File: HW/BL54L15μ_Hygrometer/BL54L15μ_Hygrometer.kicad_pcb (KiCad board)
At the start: 2 copper layers, 25.4 x 25.4 mm, 21 parts, among them IC1 nrf54L 453-00223R, J1 Conn_Qwiic, J2 Conn_ARM_JTAG_SWD_10, U1 nPM2100-QEXX, U2 SHT4x, U3 STCC4-D-R3, U5 BME688, X1 32.768 kHz

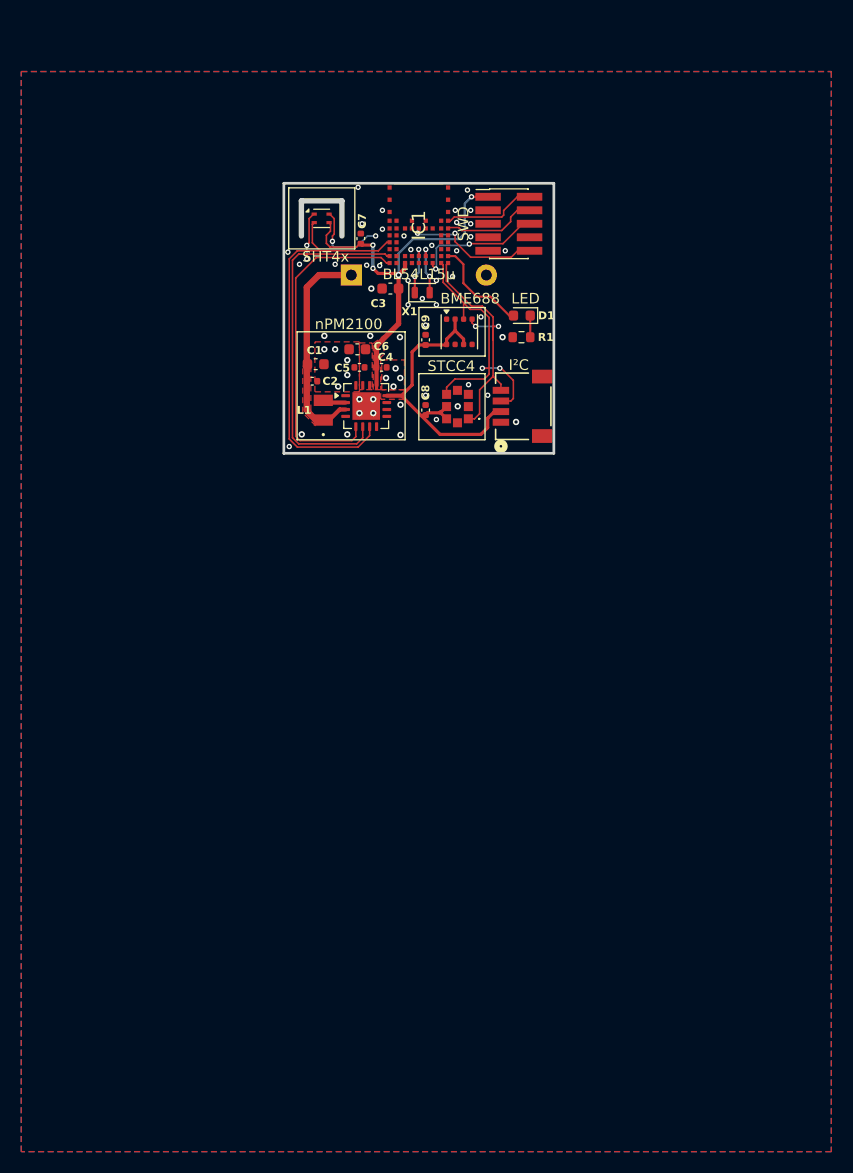
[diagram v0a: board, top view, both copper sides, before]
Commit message: BL54L15μ Hygrometer 2026v3
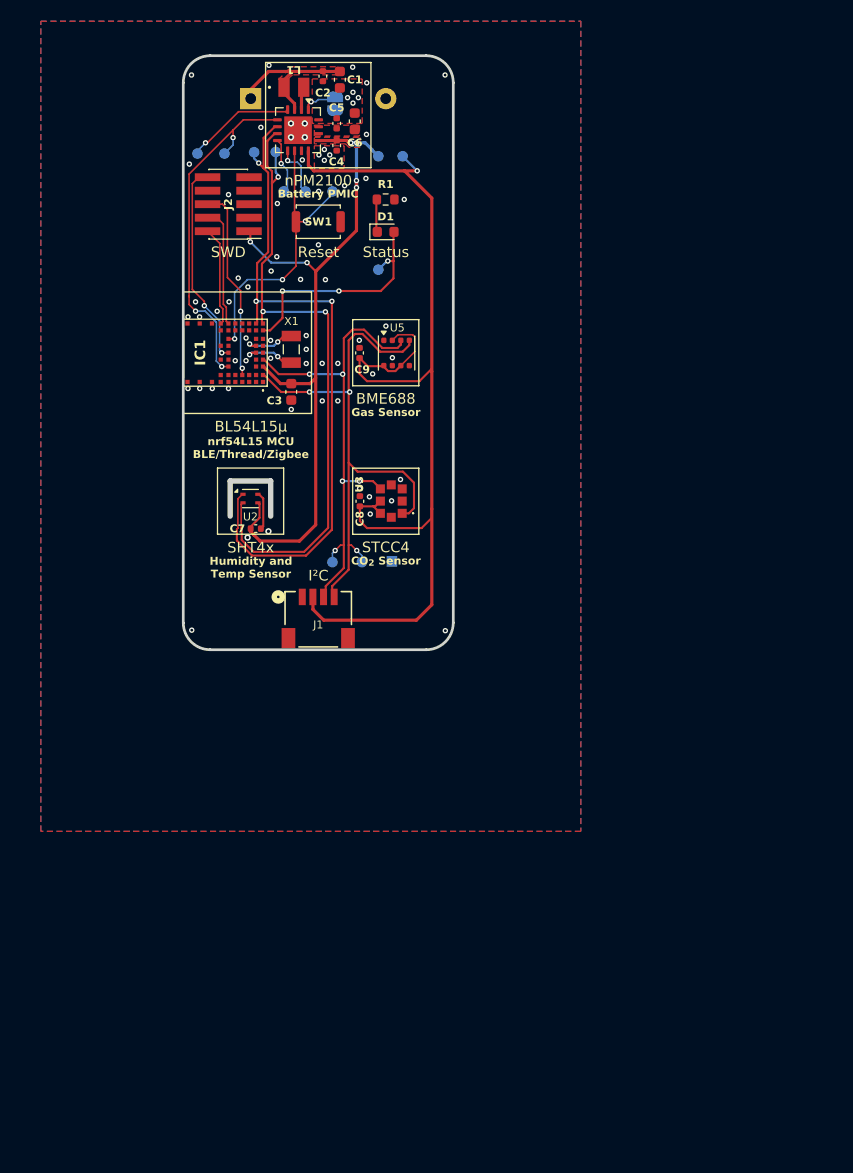
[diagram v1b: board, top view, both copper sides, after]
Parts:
- added JP1: VSET-GND, Jumper:SolderJumper-2_P1.3mm_Open_RoundedPad1.0x1.5mm, B.Cu at (103.9, 58.6)
- added SW1: Reset, Button_Switch_SMD:SW_Push_SPST_NO_Alps_SKRK, F.Cu at (102.3, 69.7)
- added TP1: VDD, TestPoint:TestPoint_Pad_D1.0mm, B.Cu at (108.0, 63.5)
- added TP10: PG/RESET, TestPoint:TestPoint_Pad_D1.0mm, B.Cu at (103.6, 66.8)
- added TP11: SYSGDEN, TestPoint:TestPoint_Pad_D1.0mm, B.Cu at (99.1, 66.8)
- added TP12: LED0, TestPoint:TestPoint_Pad_D1.0mm, B.Cu at (108.0, 74.2)
- added TP13: VDDSW, TestPoint:TestPoint_Pad_D1.0mm, B.Cu at (110.2, 63.5)
- added TP2: GND, TestPoint:TestPoint_Pad_1.0x1.0mm, B.Cu at (109.2, 101.6)
- added TP3: GPIO0/P0.01, TestPoint:TestPoint_Pad_D1.0mm, B.Cu at (93.5, 63.2)
- added TP4: GPIO1, TestPoint:TestPoint_Pad_D1.0mm, B.Cu at (101.1, 66.8)
- added TP5: SDA0/P1.14, TestPoint:TestPoint_Pad_D1.0mm, B.Cu at (96.3, 63.1)
- added TP6: SCL0/P1.04, TestPoint:TestPoint_Pad_D1.0mm, B.Cu at (98.3, 63.1)
- added TP7: SDA1/P1.06, TestPoint:TestPoint_Pad_D1.0mm, B.Cu at (103.6, 101.7)
- added TP8: SCL1/P1.08, TestPoint:TestPoint_Pad_D1.0mm, B.Cu at (106.4, 101.7)
- added TP9: SHPHLD, TestPoint:TestPoint_Pad_D1.0mm, B.Cu at (90.9, 63.2)
- BT1: footprint Battery:BatteryHolder_Keystone_2468_2xAAA -> BatteryHolder_Keystone_2468_2xAAA_NoHoles:BatteryHolder_Keystone_2468_2xAAA
- C1, C6: value 22μF -> 10μF
- IC1: footprint Ezurio 453-00223R:45300223R -> 453-00223R:45300223R
- X1: footprint Crystal:Crystal_SMD_2012-2Pin_2.0x1.2mm -> CM7V_T1A_LOW_ESR_32_768KHZ_9PF_20_TA_QC:XTAL_CM7V-T1A-LOW-ESR-32.768KHZ-9PF-20-TA-QC
- moved L1 30.5 mm to (100.0, 57.0), turned to 0 degrees
- moved C7 29.0 mm to (96.4, 98.5), turned to 0 degrees
- moved C2 28.7 mm to (102.7, 56.0), turned to -90 degrees
- moved J1 27.8 mm to (102.3, 107.1), turned to 180 degrees
- moved IC1 27.3 mm to (89.6, 82.0), turned to 180 degrees
- moved U2 27.2 mm to (95.9, 95.7)
- moved C1 26.9 mm to (104.3, 56.3), turned to -90 degrees
- moved U1 26.7 mm to (100.4, 61.0), turned to -90 degrees
- moved J2 26.5 mm to (93.8, 68.0), turned to 180 degrees
- moved C5 23.0 mm to (104.0, 60.4), turned to 90 degrees
- moved C6 21.4 mm to (105.7, 60.2), turned to 90 degrees
- moved C4 21.3 mm to (104.0, 62.5), turned to -90 degrees
- moved BT1 19.1 mm to (95.9, 58.1)
- moved R1 18.2 mm to (108.6, 67.6), turned to 0 degrees
- moved D1 15.0 mm to (108.6, 70.6), turned to 0 degrees
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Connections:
- net /NRESET renamed /~{RESET}
- D1 pad 2: /LED -> /LED0
- IC1 pad 1: /GPIO0 -> unconnected-(IC1-P2.05-Pad1)
- IC1 pad 13: /SWO -> unconnected-(IC1-P2.02-Pad13)
- IC1 pad 15: /SDA2 -> /LED0
- IC1 pad 17: /SCL2 -> /SCL0
- IC1 pad 18: /LED -> /SDA0
- IC1 pad 2: /SDA1 -> unconnected-(IC1-P2.00-Pad2)
- IC1 pad 29: unconnected-(IC1-P0.04/CLK-Pad29) -> /PG/RESET
- IC1 pad 3: unconnected-(IC1-P1.08/EXTREF/CLK16M/CLK-Pad3) -> /SCL1
- IC1 pad 35: unconnected-(IC1-P0.01-Pad35) -> /GPIO0
- IC1 pad 42: unconnected-(IC1-P2.07-Pad42) -> /SWO
- IC1 pad 43: /SCL1 -> unconnected-(IC1-P2.06/CLK-Pad43)
- IC1 pad 7: unconnected-(IC1-P1.06-Pad7) -> /SDA1
- J1 pad 3: /SDA2 -> /SDA1
- J1 pad 4: /SCL2 -> /SCL1
- U1 pad 1: unconnected-(U1-VSET-Pad1) -> /VSET
- U1 pad 10: unconnected-(U1-PG/RESET-Pad10) -> /PG/RESET
- U1 pad 4: unconnected-(U1-SHPHLD-Pad4) -> /SHPHLD
- U1 pad 6: /SDA1 -> /SDA0
- U1 pad 7: /SCL1 -> /SCL0
- U1 pad 8: unconnected-(U1-SYSGDEN-Pad8) -> /SYSGDEN
- U1 pad 9: unconnected-(U1-GPIO1-Pad9) -> /GPIO1
- U2 pad 1: /SDA1 -> /SDA0
- U2 pad 2: /SCL1 -> /SCL0
- U3 pad 1: /SCL2 -> /SCL1
- U3 pad 5: /SDA2 -> /SDA1
- U5 pad 3: /SDA2 -> /SDA1
- U5 pad 4: /SCL2 -> /SCL1
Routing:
- net VDDSW: track 29.7 -> 101.4 mm, vias 0 -> 1
- net /SDA0: track 0.00 -> 65.3 mm, vias 0 -> 3
- net /SCL0: track 0.00 -> 61.9 mm, vias 0 -> 3
- net VDD: track 38.7 -> 69.3 mm, vias 4 -> 6
- net /PG/RESET: track 0.00 -> 27.4 mm, vias 0 -> 3
- net /SDA2: track 26.6 -> 0.00 mm, vias 2 -> 0
- net /SCL2: track 24.8 -> 0.00 mm, vias 2 -> 0
- net /LED0: track 0.00 -> 21.9 mm, vias 0 -> 3
- net /SCL1: track 39.3 -> 53.9 mm, vias 0 -> 3
- net /SHPHLD: track 0.00 -> 10.3 mm, vias 0 -> 1
- net /LED: track 9.51 -> 0.00 mm
- net /VBAT: track 20.6 -> 12.9 mm
- net /SDA1: track 39.3 -> 46.1 mm, vias 2 -> 5
- net /SWO: track 12.4 -> 18.2 mm
- net /~{RESET}: track 12.8 -> 18.6 mm
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- removed copper zone on F.Cu, net VDDSW
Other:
- board size 25.4 x 25.4 mm -> 25.4 x 55.9 mm
- board text added: "${TITLE} nRF54L15 MCU"
- board text added: "BME688 Pressure/Gas I²C 0x76 P1.06/P1.08"
- board text added: "Battery PMIC"
- board text added: "CO_{2} Sensor"
- board text added: "Gas Sensor"
- board text added: "Hot loop: VBAT -> SW -> VINT -> PVSS (VBAT GND)"
- board text added: "Humidity and Temp Sensor"
- board text added: "I²C Connector STEMMA QT SDA P1.06 SCL P1.08 Load switched"
- board text added: "I²C0 SDA P1.14 SCL P1.04 I²C1 SDA P1.06 SCL P1.08 I²C0 VDD, I²C1 nPM2100 LS MCU 13k pull-ups required"
- board text added: "Reset"
- board text added: "SHT4x Humidity/temp I²C 0x44 P1.14/P1.04 Thermal cutout"
- board text added: "STCC4 CO₂±(100 ppm + 10%) I²C 0x64 P1.06/P1.08"
- board text added: "Status"
- board text added: "nPM2100 I²C 0x74 SDA P1.14 SCL P1.04"
- board text added: "nrf54L15 MCU BLE/Thread/Zigbee"
- board text removed: "BL54L15μ: nrf54L15 MCU module nPM2100: bat .7-3.4V, I2C1 0x74 SHT4x: Humidity/temp, I2C1 0x44 STCC4: C02, min 2.7V, I2C2 0x64 BME688: Pressure/Gas, I2C2 0x76 Qwiic I2C receptable on bus 2"
- board text removed: "LED"
